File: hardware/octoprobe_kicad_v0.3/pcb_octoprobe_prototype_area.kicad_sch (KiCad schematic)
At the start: 15 parts, among them J1101 Conn_01x20, J1102 Conn_01x20, J1103 Conn_01x20

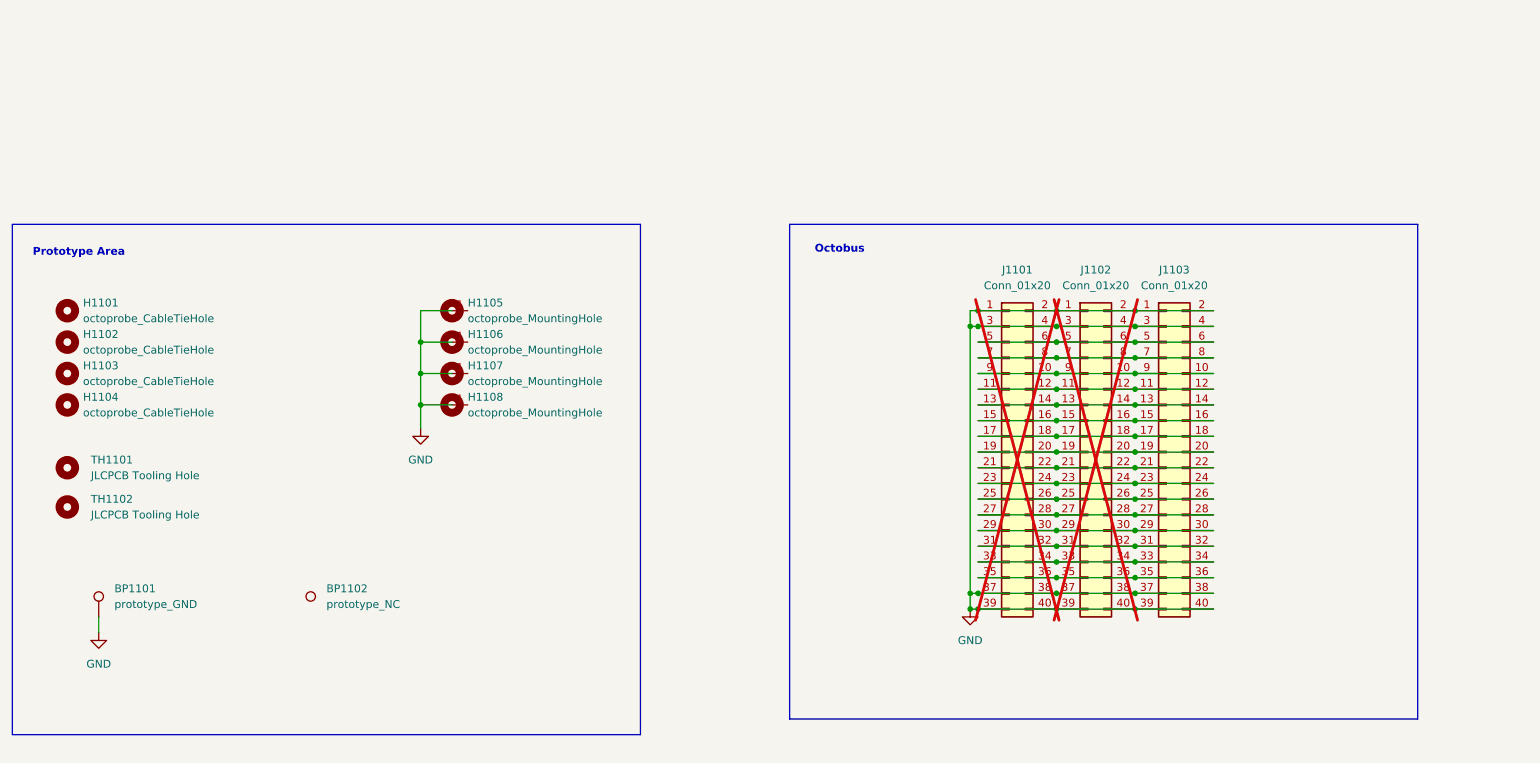
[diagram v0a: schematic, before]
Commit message: PCB: Octobus
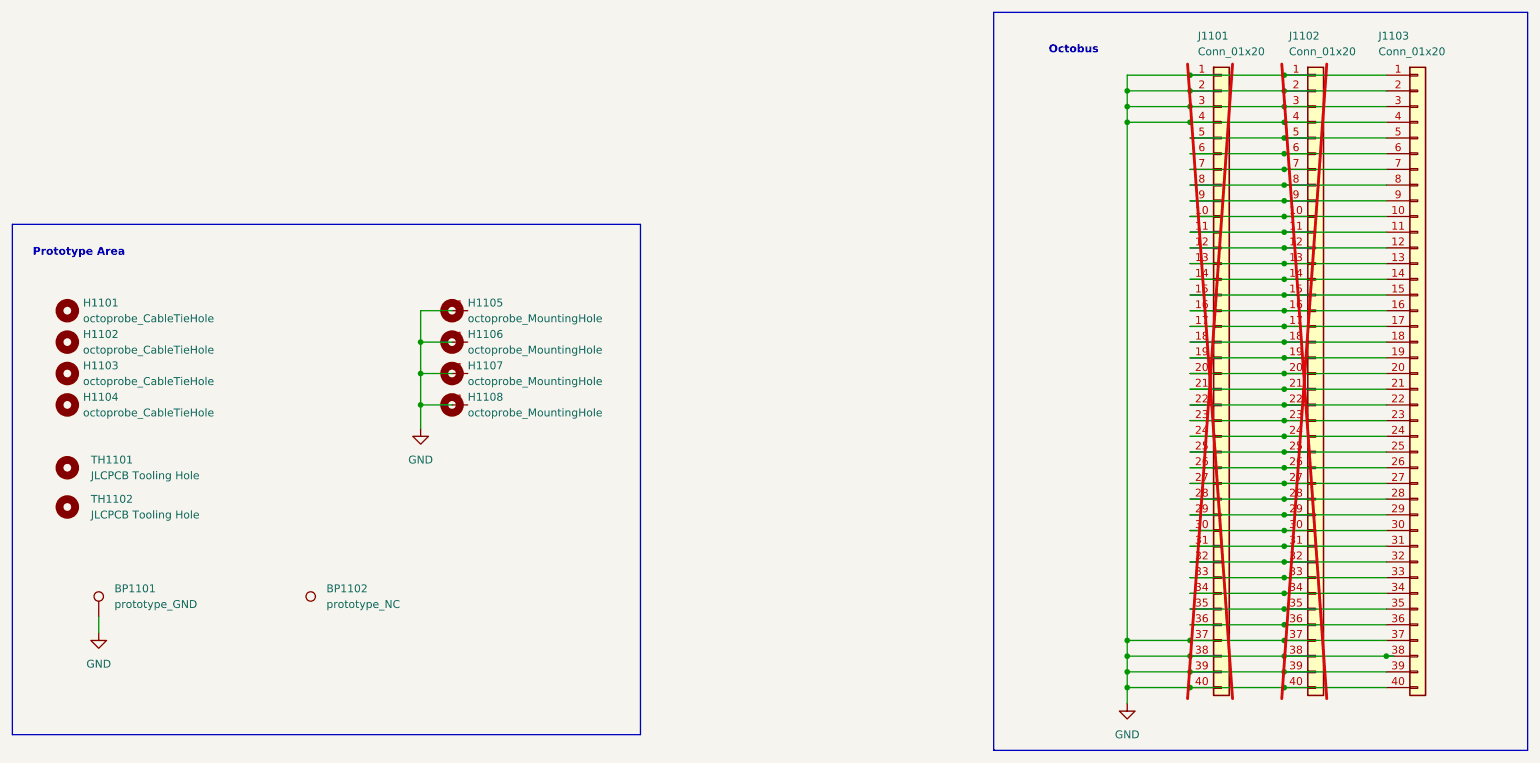
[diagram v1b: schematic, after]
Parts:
- J1101, J1102, J1103: footprint 00_project_library:PinSocket_2x20_P2.54mm_Vertical-mirrored-stackable -> 00_project_library:PinSocket_2x20_P2.54mm_Vertical-stackable_squarepad; symbol Connector_Generic:Conn_02x20_Odd_Even -> Connector_Generic:Conn_01x40; now in the parts list
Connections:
- net at J1101.10 (Pin_10), J1102.10 (Pin_10), J1103.10 (Pin_10): no longer J1101.9 (Pin_9), J1102.9 (Pin_9), J1103.9 (Pin_9)
- net at J1101.11 (Pin_11), J1102.11 (Pin_11), J1103.11 (Pin_11): no longer J1101.12 (Pin_12), J1102.12 (Pin_12), J1103.12 (Pin_12)
- net at J1101.13 (Pin_13), J1102.13 (Pin_13), J1103.13 (Pin_13): no longer J1101.14 (Pin_14), J1102.14 (Pin_14), J1103.14 (Pin_14)
- net at J1101.15 (Pin_15), J1102.15 (Pin_15), J1103.15 (Pin_15): no longer J1101.16 (Pin_16), J1102.16 (Pin_16), J1103.16 (Pin_16)
- net at J1101.17 (Pin_17), J1102.17 (Pin_17), J1103.17 (Pin_17): no longer J1101.18 (Pin_18), J1102.18 (Pin_18), J1103.18 (Pin_18)
- net at J1101.19 (Pin_19), J1102.19 (Pin_19), J1103.19 (Pin_19): no longer J1101.20 (Pin_20), J1102.20 (Pin_20), J1103.20 (Pin_20)
- net at J1101.21 (Pin_21), J1102.21 (Pin_21), J1103.21 (Pin_21): no longer J1101.22 (Pin_22), J1102.22 (Pin_22), J1103.22 (Pin_22)
- net at J1101.23 (Pin_23), J1102.23 (Pin_23), J1103.23 (Pin_23): no longer J1101.24 (Pin_24), J1102.24 (Pin_24), J1103.24 (Pin_24)
- net at J1101.25 (Pin_25), J1102.25 (Pin_25), J1103.25 (Pin_25): no longer J1101.26 (Pin_26), J1102.26 (Pin_26), J1103.26 (Pin_26)
- net at J1101.27 (Pin_27), J1102.27 (Pin_27), J1103.27 (Pin_27): no longer J1101.28 (Pin_28), J1102.28 (Pin_28), J1103.28 (Pin_28)
- net at J1101.29 (Pin_29), J1102.29 (Pin_29), J1103.29 (Pin_29): no longer J1101.30 (Pin_30), J1102.30 (Pin_30), J1103.30 (Pin_30)
- net at J1101.31 (Pin_31), J1102.31 (Pin_31), J1103.31 (Pin_31): no longer J1101.32 (Pin_32), J1102.32 (Pin_32), J1103.32 (Pin_32)
- net at J1101.33 (Pin_33), J1102.33 (Pin_33), J1103.33 (Pin_33): no longer J1101.34 (Pin_34), J1102.34 (Pin_34), J1103.34 (Pin_34)
- net at J1101.35 (Pin_35), J1102.35 (Pin_35), J1103.35 (Pin_35): no longer J1101.36 (Pin_36), J1102.36 (Pin_36), J1103.36 (Pin_36)
- net at J1101.5 (Pin_5), J1102.5 (Pin_5), J1103.5 (Pin_5): no longer J1101.6 (Pin_6), J1102.6 (Pin_6), J1103.6 (Pin_6)
- net at J1101.7 (Pin_7), J1102.7 (Pin_7), J1103.7 (Pin_7): no longer J1101.8 (Pin_8), J1102.8 (Pin_8), J1103.8 (Pin_8)
- new net: J1101.12 (Pin_12), J1102.12 (Pin_12), J1103.12 (Pin_12)
- new net: J1101.14 (Pin_14), J1102.14 (Pin_14), J1103.14 (Pin_14)
- new net: J1101.16 (Pin_16), J1102.16 (Pin_16), J1103.16 (Pin_16)
- new net: J1101.18 (Pin_18), J1102.18 (Pin_18), J1103.18 (Pin_18)
- new net: J1101.20 (Pin_20), J1102.20 (Pin_20), J1103.20 (Pin_20)
- new net: J1101.22 (Pin_22), J1102.22 (Pin_22), J1103.22 (Pin_22)
- new net: J1101.24 (Pin_24), J1102.24 (Pin_24), J1103.24 (Pin_24)
- new net: J1101.26 (Pin_26), J1102.26 (Pin_26), J1103.26 (Pin_26)
- new net: J1101.28 (Pin_28), J1102.28 (Pin_28), J1103.28 (Pin_28)
- new net: J1101.30 (Pin_30), J1102.30 (Pin_30), J1103.30 (Pin_30)
- new net: J1101.32 (Pin_32), J1102.32 (Pin_32), J1103.32 (Pin_32)
- new net: J1101.34 (Pin_34), J1102.34 (Pin_34), J1103.34 (Pin_34)
- new net: J1101.36 (Pin_36), J1102.36 (Pin_36), J1103.36 (Pin_36)
- new net: J1101.6 (Pin_6), J1102.6 (Pin_6), J1103.6 (Pin_6)
- new net: J1101.8 (Pin_8), J1102.8 (Pin_8), J1103.8 (Pin_8)
- new net: J1101.9 (Pin_9), J1102.9 (Pin_9), J1103.9 (Pin_9)
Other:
- moved on the sheet: J1101, J1102, J1103
